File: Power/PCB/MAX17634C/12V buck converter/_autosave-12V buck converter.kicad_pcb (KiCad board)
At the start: 32 copper layers, 24.5 x 24.5 mm, 11 parts, among them IC1 MAX17634C

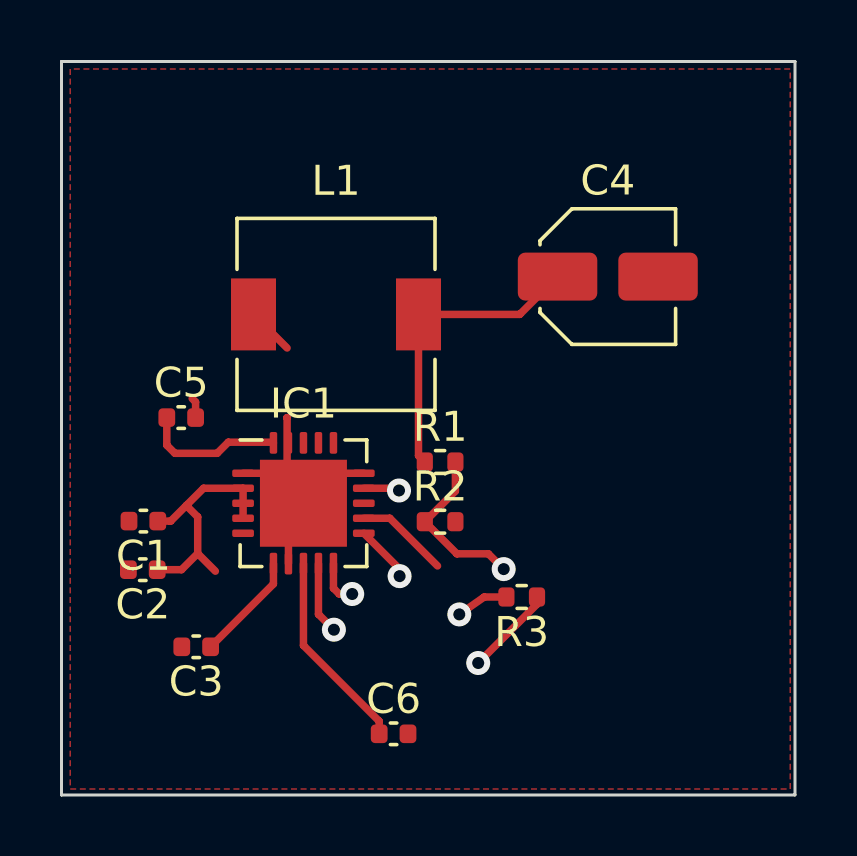
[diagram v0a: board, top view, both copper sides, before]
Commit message: PS drawio IC update
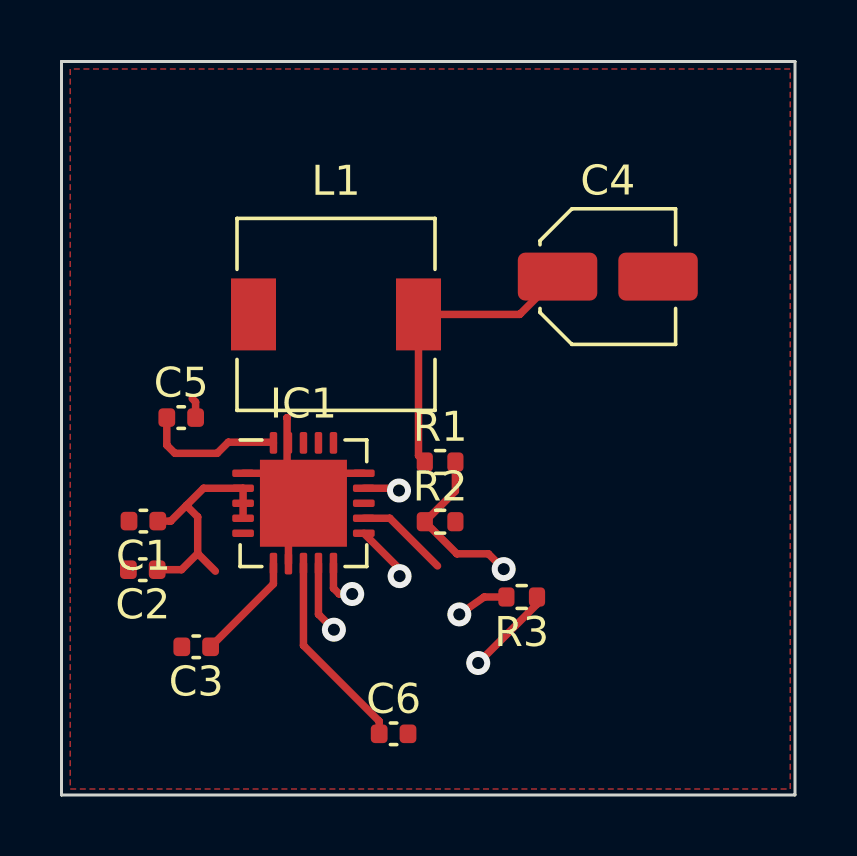
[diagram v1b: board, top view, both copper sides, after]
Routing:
- net Earth: track 15.1 -> 13.5 mm
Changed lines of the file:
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@@
     (fp_line (start 0.5 0.25) (end -0.5 0.25)
       (stroke (width 0.1) (type solid)) (layer "F.Fab"))
-    (pad "1" smd roundrect locked (at -0.48 0 180) (size 0.56 0.62) (layers "F.Cu" "F.Paste" "F.Mask") (roundrect_rratio 0.25)
+    (pad "1" smd roundrect (at -0.48 0 180) (size 0.56 0.62) (layers "F.Cu" "F.Paste" "F.Mask") (roundrect_rratio 0.25)
       (net 1 "Net-(IC1-EN{slash}UVLO)") (pintype "passive"))
     (pad "2" smd roundrect (at 0.48 0 180) (size 0.56 0.62) (layers "F.Cu" "F.Paste" "F.Mask") (roundrect_rratio 0.25)
@@
   (segment (start 108.18 62.6) (end 108.18 63.12) (width 0.25) (layer "F.Cu") (net 2))
   (segment (start 111.22 63.12) (end 111.23 63.13) (width 0.25) (layer "F.Cu") (net 2))
-  (segment (start 110.11 59.68) (end 111.23 60.8) (width 0.25) (layer "F.Cu") (net 2))
   (segment (start 108.065 62.485) (end 108.18 62.6) (width 0.25) (layer "F.Cu") (net 2))
   (segment (start 113.7875 64.975) (end 112.775 64.975) (width 0.25) (layer "F.Cu") (net 2))
